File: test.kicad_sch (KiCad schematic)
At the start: 15 parts, among them U1 ATmega8L-8P, U2 74AHC595, U3 74AHC595, U4 74AHC595, U5 74AHC595, Y1 8 MHz Crystal

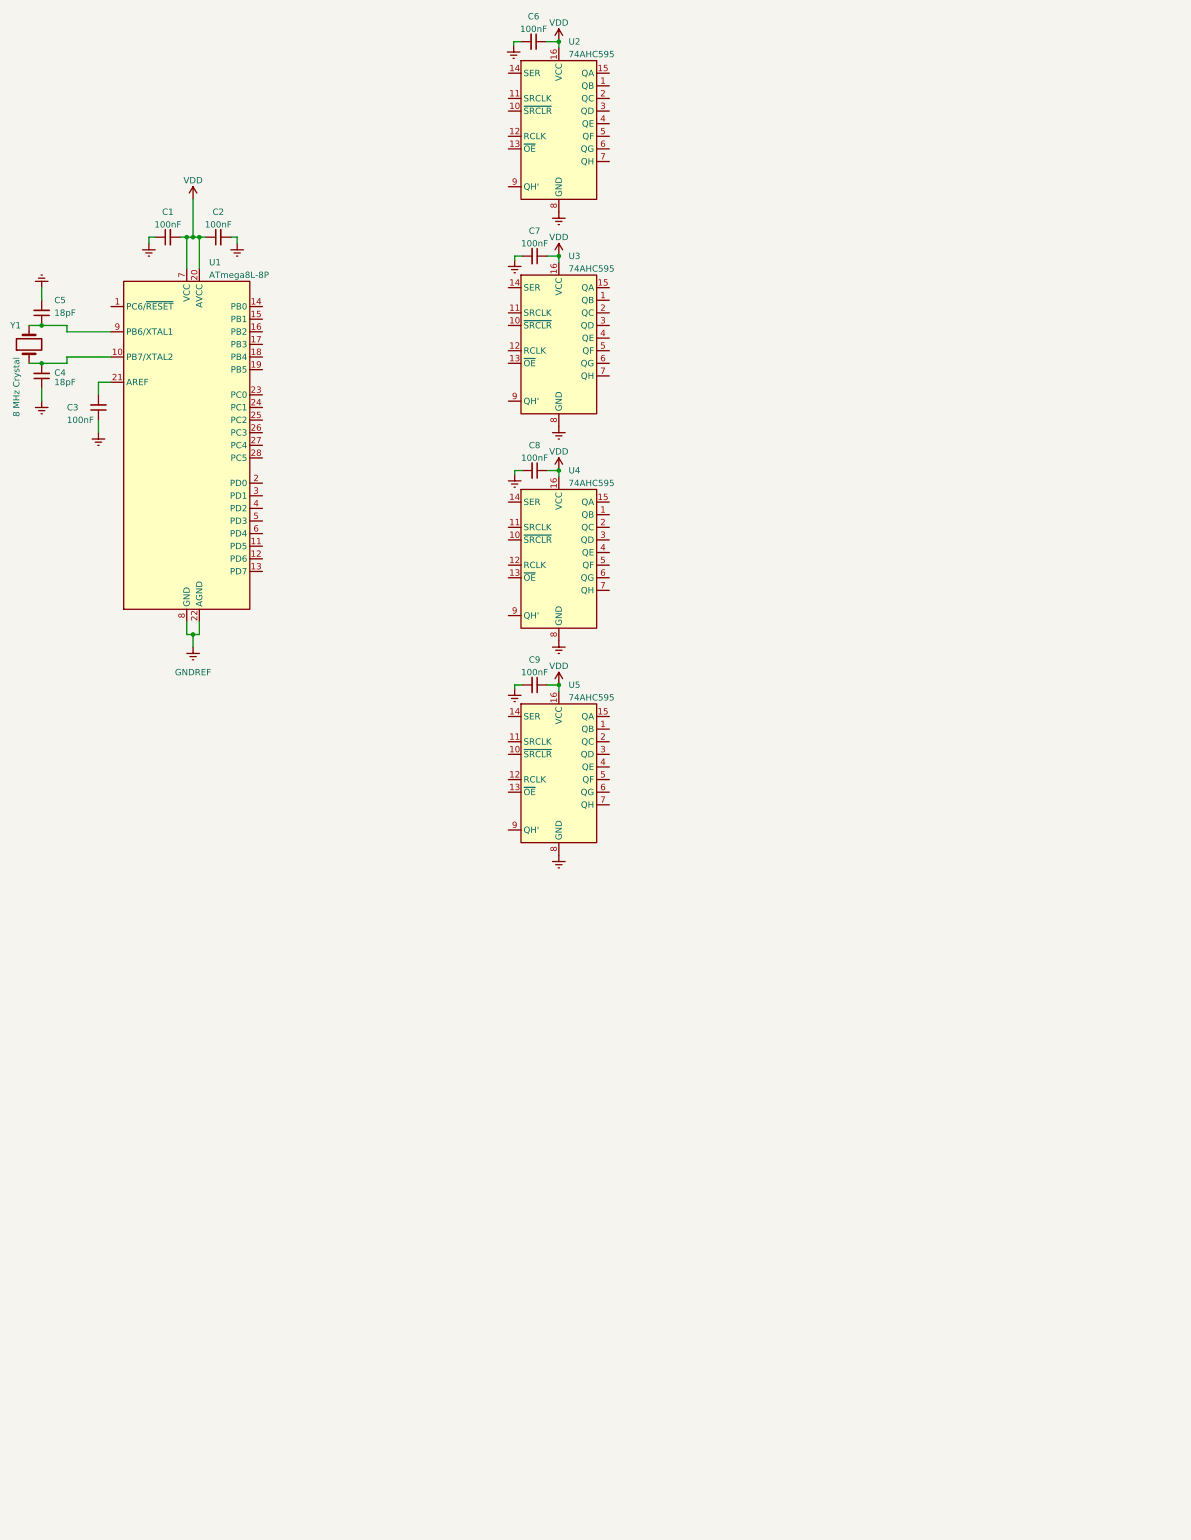
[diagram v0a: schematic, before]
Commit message: add some more stuff
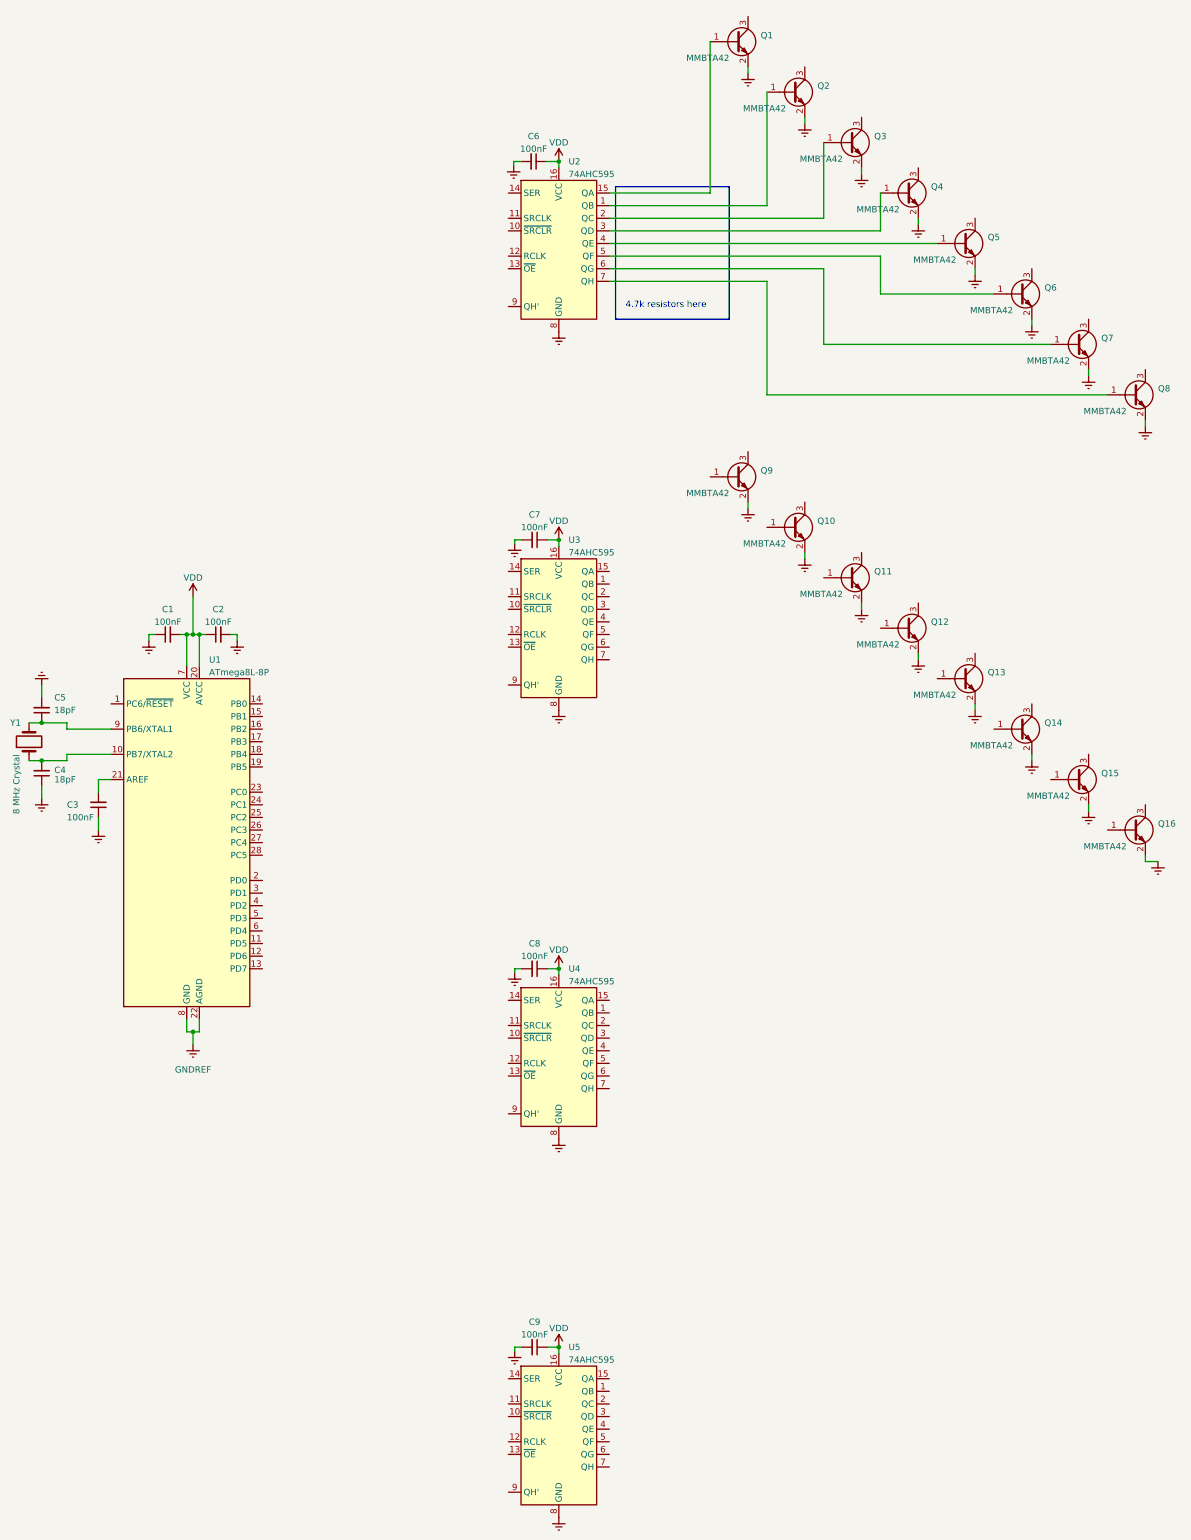
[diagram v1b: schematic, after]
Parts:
- added Q1, Q10, Q11, Q12, Q13, Q14, Q15, Q16, Q2, Q3, Q4, Q5, Q6, Q7, Q8, Q9: MMBTA42, Package_TO_SOT_SMD:SOT-23W_Handsoldering, symbol Transistor_BJT:MMBTA42
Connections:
- net GNDREF: now also Q1.2 (E), Q10.2 (E), Q11.2 (E), Q12.2 (E), Q13.2 (E), Q14.2 (E), Q15.2 (E), Q16.2 (E), Q2.2 (E), Q3.2 (E), Q4.2 (E), Q5.2 (E), Q6.2 (E), Q7.2 (E), Q8.2 (E), Q9.2 (E)
- net at U2.1 (QB): now also Q2.1 (B)
- net at U2.15 (QA): now also Q1.1 (B)
- net at U2.2 (QC): now also Q3.1 (B)
- net at U2.3 (QD): now also Q4.1 (B)
- net at U2.4 (QE): now also Q5.1 (B)
- net at U2.5 (QF): now also Q6.1 (B)
- net at U2.6 (QG): now also Q7.1 (B)
- net at U2.7 (QH): now also Q8.1 (B)
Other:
- note added: "4.7k resistors here"
- moved on the sheet: C1, C2, C3, C4, C5, C6, C7, C8, C9, U1, U2, U3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
